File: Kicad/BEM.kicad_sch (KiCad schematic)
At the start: 17 parts, among them U2 ACS712xLCTR-30A, U3 ACS712xLCTR-30A, U4 ACS712xLCTR-30A, U5 ACS712xLCTR-30A

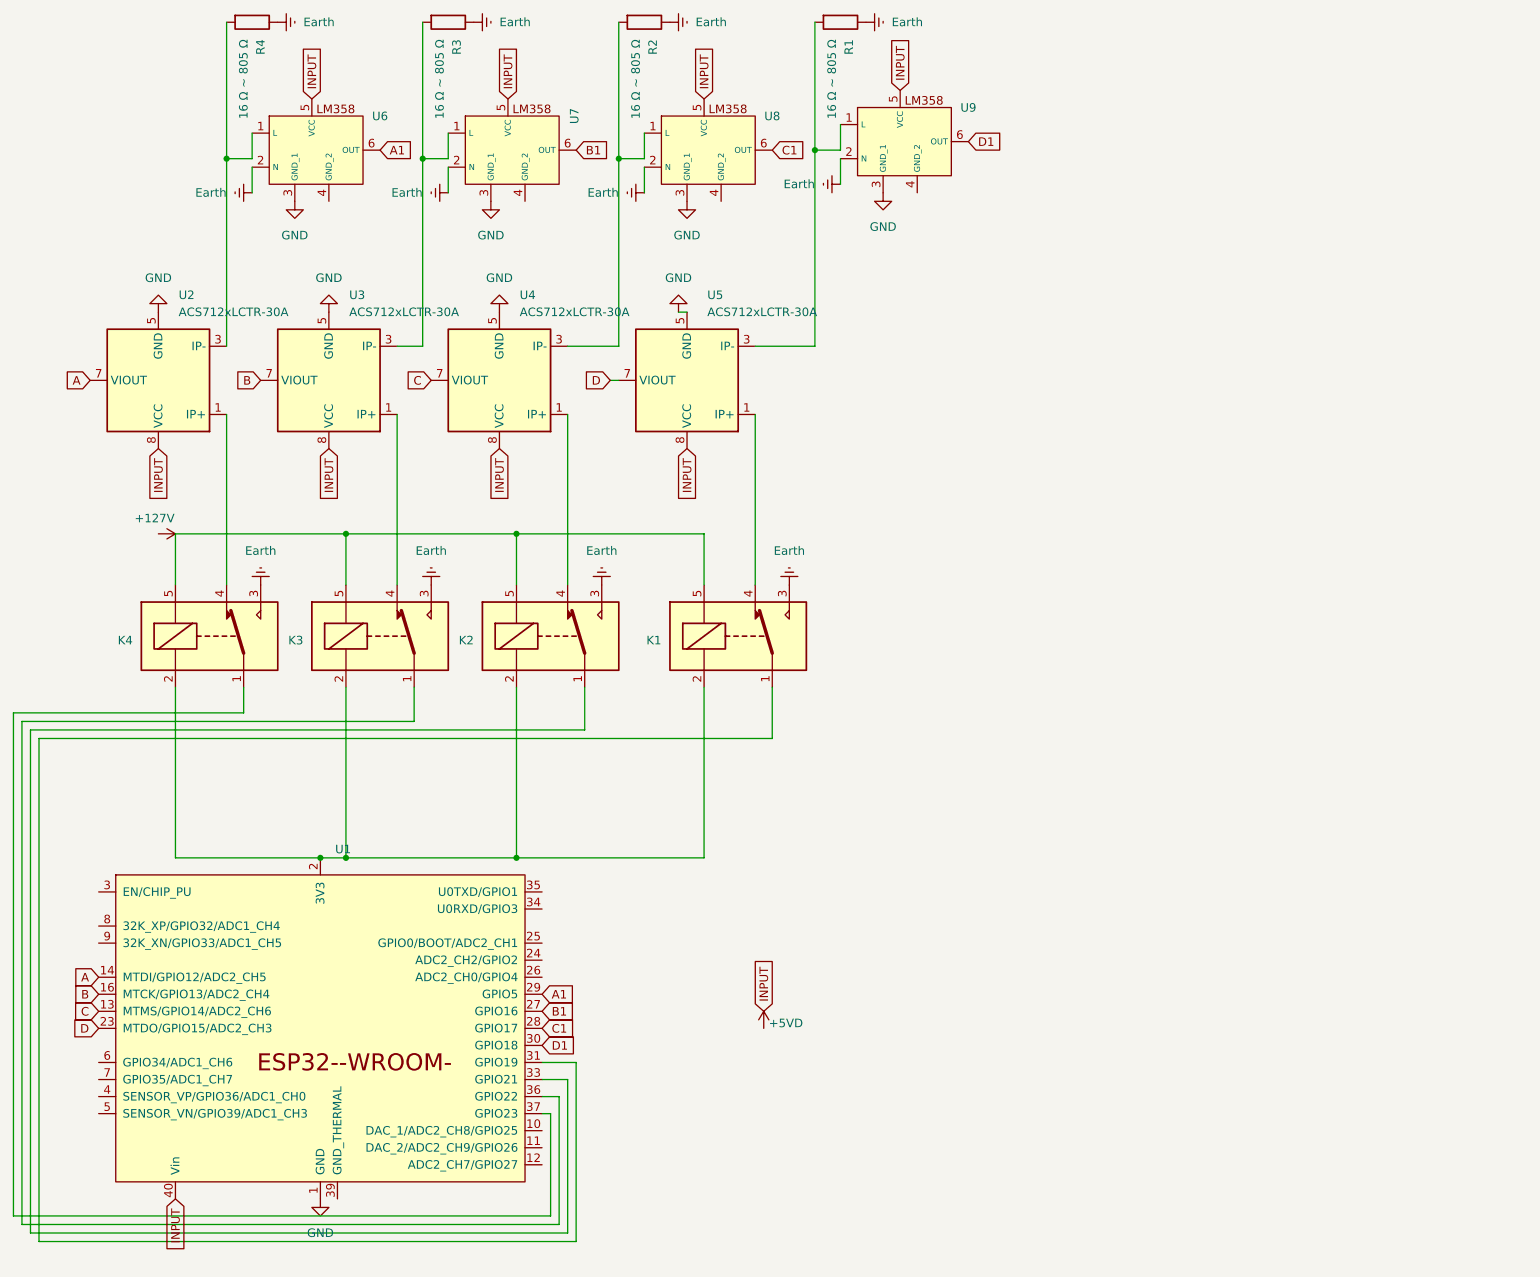
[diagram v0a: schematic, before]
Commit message: Added: Schem V2, Schem.png
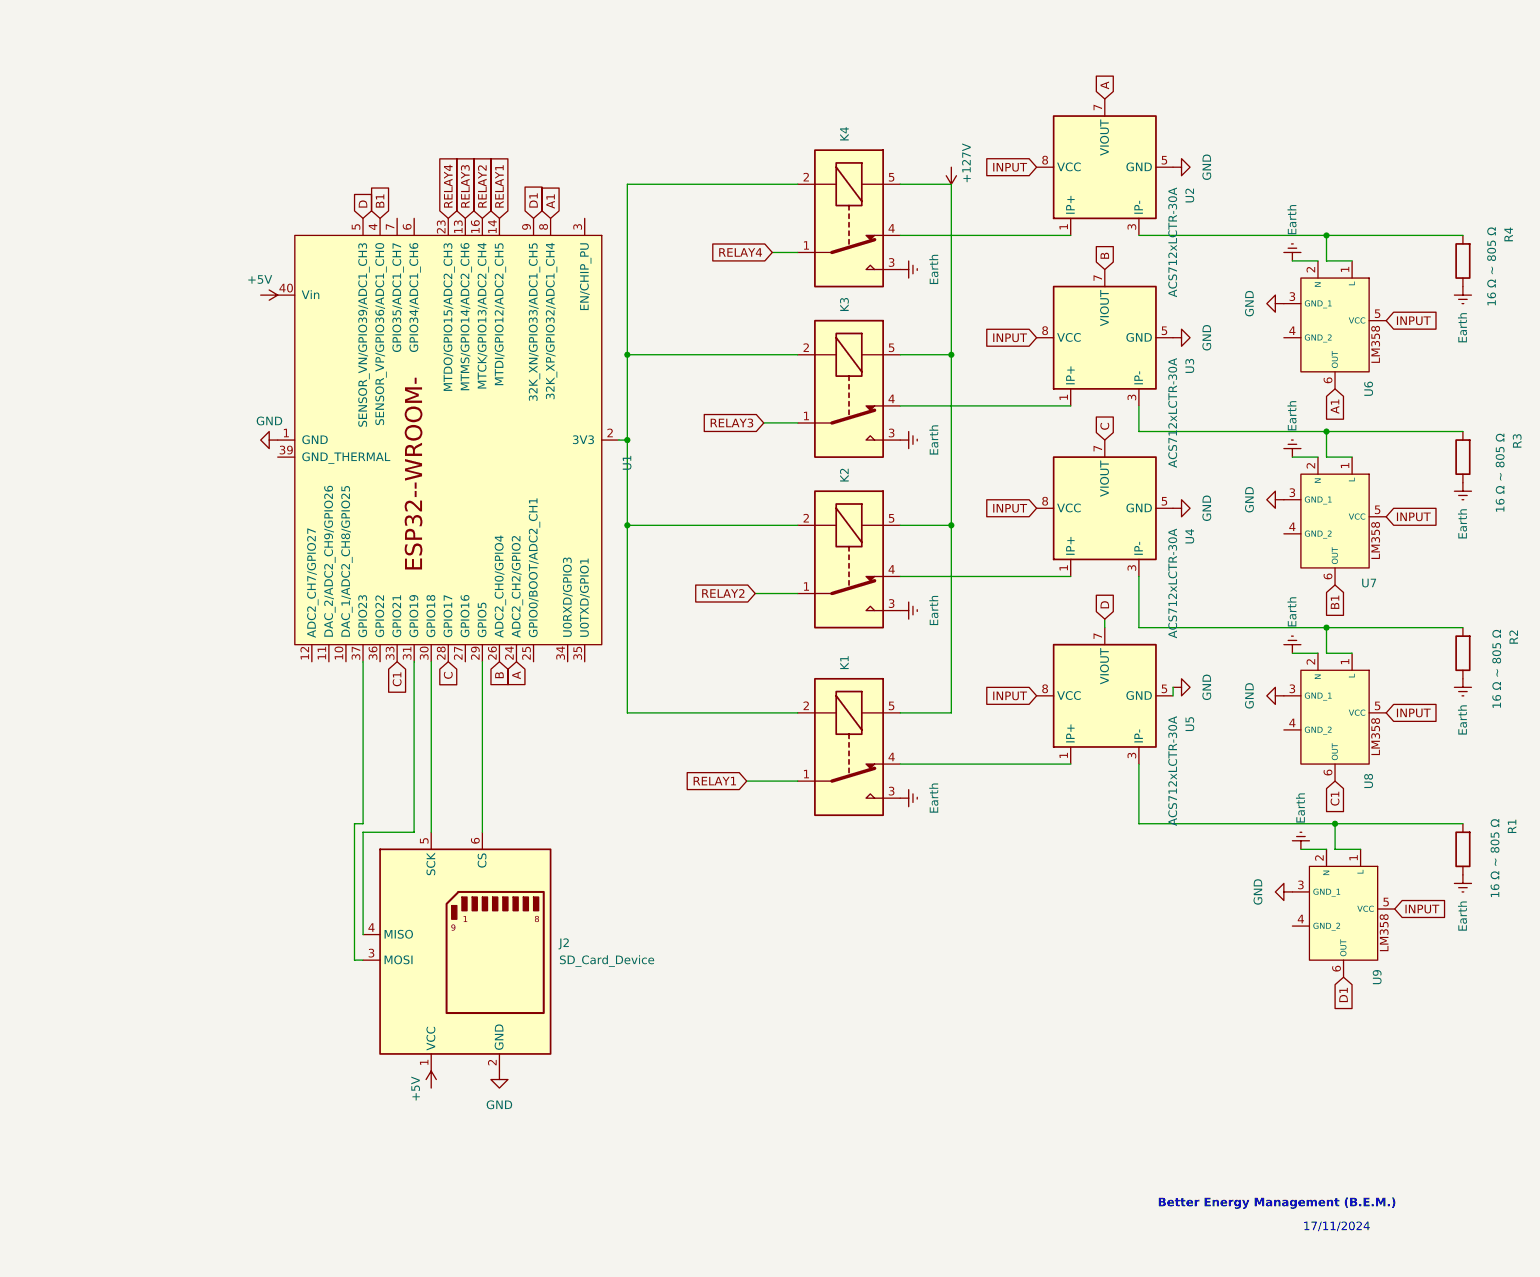
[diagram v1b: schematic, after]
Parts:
- added J2: SD_Card_Device, symbol Connector:SD_Card_Device
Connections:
- net A: now also U1.24 (ADC2_CH2/GPIO2); no longer U1.14 (MTDI/GPIO12/ADC2_CH5)
- net A1: now also U1.8 (32K_XP/GPIO32/ADC1_CH4); no longer U1.29 (GPIO5)
- net B: now also U1.26 (ADC2_CH0/GPIO4); no longer U1.16 (MTCK/GPIO13/ADC2_CH4)
- net B1: now also U1.4 (SENSOR_VP/GPIO36/ADC1_CH0); no longer U1.27 (GPIO16)
- net C: now also U1.28 (GPIO17); no longer U1.13 (MTMS/GPIO14/ADC2_CH6)
- net C1: now also U1.33 (GPIO21); no longer U1.28 (GPIO17)
- net D: now also U1.5 (SENSOR_VN/GPIO39/ADC1_CH3); no longer U1.23 (MTDO/GPIO15/ADC2_CH3)
- net D1: now also U1.9 (32K_XN/GPIO33/ADC1_CH5); no longer U1.30 (GPIO18)
- net GND: now also J2.2 (GND)
- net INPUT: no longer U1.40 (Vin)
- net at U1.36 (GPIO22): no longer K3.1
- net at U1.37 (GPIO23): now also J2.3 (MOSI); no longer K4.1
- net at U1.31 (GPIO19): now also J2.4 (MISO); no longer K1.1
- net RELAY2: now reaches K2.1
- net RELAY2: now also U1.16 (MTCK/GPIO13/ADC2_CH4); no longer U1.33 (GPIO21)
- new net: J2.6 (CS), U1.29 (GPIO5)
- new net: J2.5 (SCK), U1.30 (GPIO18)
- new net RELAY1: K1.1, U1.14 (MTDI/GPIO12/ADC2_CH5)
- new net RELAY3: K3.1, U1.13 (MTMS/GPIO14/ADC2_CH6)
- new net RELAY4: K4.1, U1.23 (MTDO/GPIO15/ADC2_CH3)
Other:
- note added: "17/11/2024"
- note added: "Better Energy Management (B.E.M.)"
- moved on the sheet: K1, K2, K3, K4, R1, R2, R3, R4, U1, U2, U3, U4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
